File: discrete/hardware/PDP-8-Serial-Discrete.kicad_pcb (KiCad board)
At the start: 2 copper layers, 125.2 x 61.9 mm, 103 parts, among them J1 Screw_Terminal_01x06, J2 DE9_Socket_MountingHoles, J3 FlipChip_01x18, Q1 2N5551, Q10 2N5401, Q11 2N5401, Q12 2N5551, Q13 2N5401, Q14 2N5551, Q15 2N5401, Q16 2N5551, Q17 2N5401, Q2 2N5401, Q3 2N5401, Q4 2N5401, Q5 2N5551, Q6 2N5401, Q7 2N5551, Q8 2N5401, Q9 2N5551

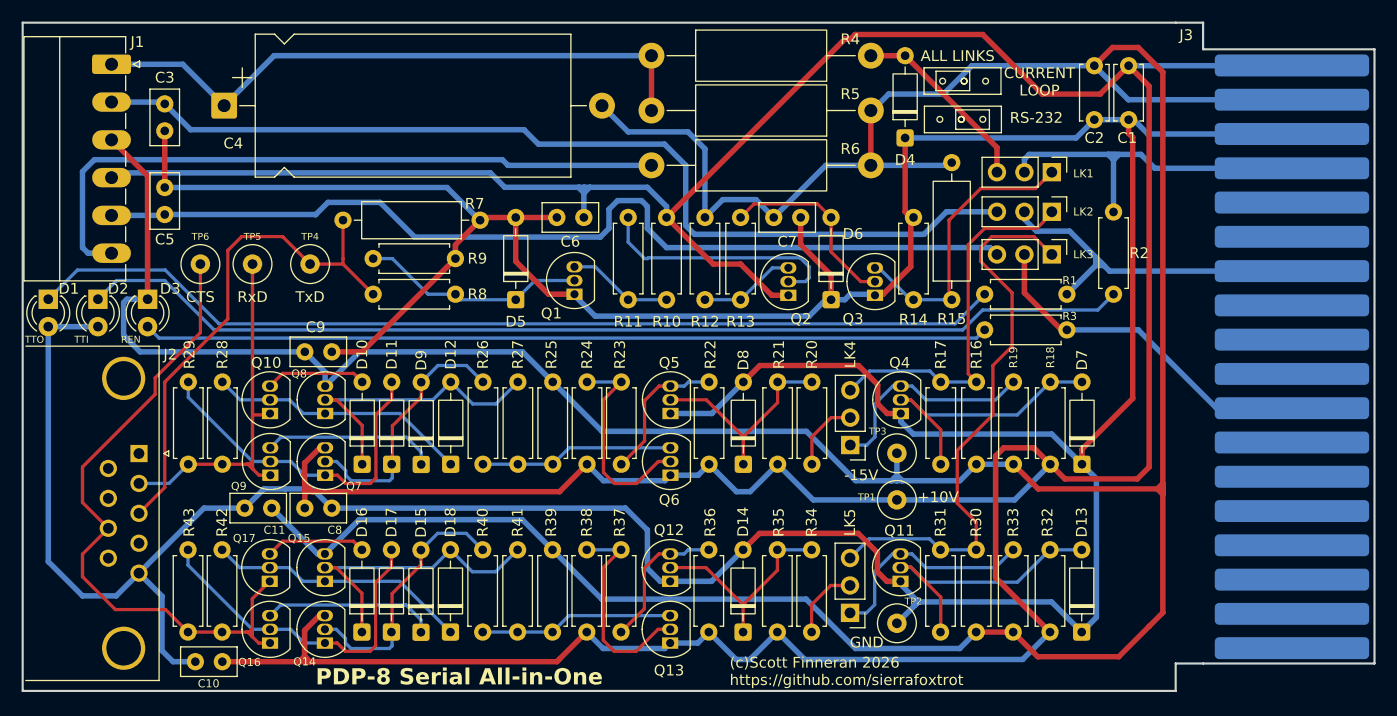
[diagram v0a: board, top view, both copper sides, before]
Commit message: PCB cleanup
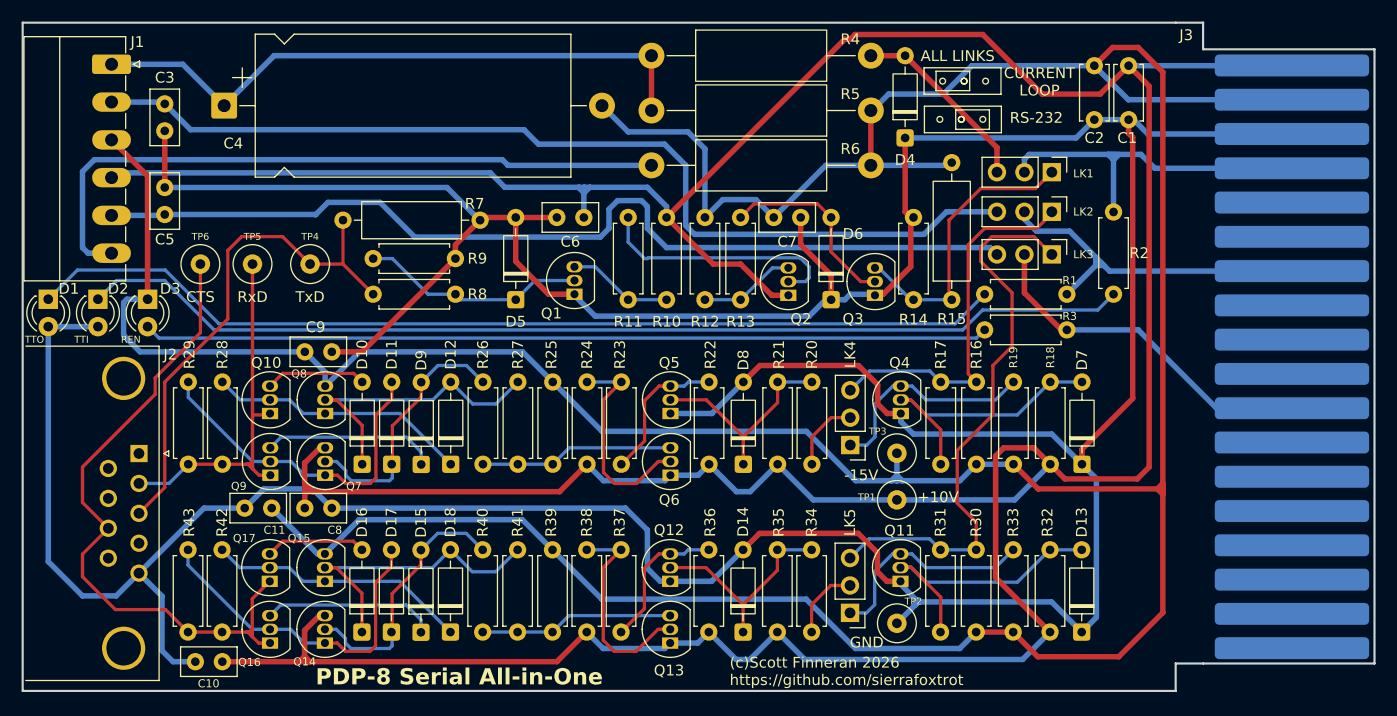
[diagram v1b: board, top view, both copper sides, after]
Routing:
- net +10V: track 388.0 -> 387.4 mm
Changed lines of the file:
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@@
 	)
 	(segment
-		(start 108.966 130.302)
-		(end 106.974 130.302)
+		(start 106.974 130.302)
+		(end 111.486 130.302)
 		(width 0.508)
 		(layer "B.Cu")
@@
 	)
 	(segment
-		(start 181.292501 126.555499)
-		(end 182.753 128.015999)
-		(width 0.508)
-		(layer "B.Cu")
-		(net 1)
-	)
-	(segment
 		(start 159.004 112.776)
 		(end 157.48 114.3)
@@
 	)
 	(segment
-		(start 181.267704 142.101005)
+		(start 179.934205 140.767506)
 		(end 182.728203 143.561505)
 		(width 0.508)
@@
 	)
 	(segment
-		(start 179.934205 140.767506)
-		(end 181.267704 142.101005)
-		(width 0.508)
-		(layer "B.Cu")
-		(net 1)
-	)
-	(segment
 		(start 140.462 132.08)
 		(end 113.264 132.08)
@@
 	)
 	(segment
-		(start 111.486 130.302)
-		(end 108.966 130.302)
-		(width 0.508)
-		(layer "B.Cu")
-		(net 1)
-	)
-	(segment
 		(start 163.322 112.268)
 		(end 161.29 112.268)
@@
 	(segment
 		(start 179.959002 125.222)
-		(end 181.292501 126.555499)
+		(end 182.753 128.015999)
 		(width 0.508)
 		(layer "B.Cu")
@@
 	)
 	(segment
-		(start 110.744 145.288)
+		(start 110.744 145.796)
 		(end 110.744 143.403274)
 		(width 0.508)
@@
 	(segment
 		(start 134.111999 146.304)
-		(end 134.365999 146.05)
+		(end 136.906 143.509999)
 		(width 0.508)
 		(layer "F.Cu")
@@
 	)
 	(segment
-		(start 110.744 145.796)
-		(end 110.744 145.288)
-		(width 0.508)
-		(layer "F.Cu")
-		(net 2)
-	)
-	(segment
 		(start 134.365999 130.556)
 		(end 111.506 130.556)
@@
 	)
 	(segment
-		(start 136.906 143.509999)
-		(end 134.365999 146.05)
-		(width 0.508)
-		(layer "F.Cu")
-		(net 2)
-	)
-	(segment
 		(start 110.744 127.909274)
 		(end 112.161275 126.491999)
@@
 	)
 	(segment
-		(start 154.559 128.015999)
-		(end 154.559 128.143)
-		(width 0.508)
-		(layer "B.Cu")
-		(net 2)
-	)
-	(segment
 		(start 142.494 102.362)
 		(end 144.272 104.14)
@@
 	)
 	(segment
-		(start 201.922 91.353)
-		(end 202.2 91.075)
-		(width 0.508)
-		(layer "B.Cu")
-		(net 2)
-	)
-	(segment
-		(start 154.534203 143.561505)
-		(end 154.534203 143.688506)
-		(width 0.508)
-		(layer "B.Cu")
-		(net 2)
-	)
-	(segment
 		(start 144.123999 129.54)
 		(end 138.430001 129.54)
@@
 	)
 	(segment
-		(start 188.976 143.028709)
-		(end 186.157203 145.847506)
-		(width 0.508)
-		(layer "F.Cu")
-		(net 3)
-	)
-	(segment
-		(start 190.246 141.758709)
-		(end 188.976 143.028709)
+		(start 186.157203 145.847506)
+		(end 190.246 141.758709)
 		(width 0.508)
 		(layer "F.Cu")
@@
 	)
 	(segment
-		(start 170.18 100.33)
-		(end 170.434 100.076)
-		(width 0.508)
-		(layer "B.Cu")
-		(net 3)
-	)
-	(segment
 		(start 187.047 94.25)
 		(end 202.2 94.25)
@@
 	)
 	(segment
-		(start 124.46 120.395999)
-		(end 124.46 120.65)
-		(width 0.3048)
-		(layer "F.Cu")
-		(net 12)
-	)
-	(segment
 		(start 116.078 124.421199)
 		(end 113.7038 122.046999)
@@
 	)
 	(segment
-		(start 124.435203 135.941505)
-		(end 124.435203 136.195506)
-		(width 0.3048)
-		(layer "F.Cu")
-		(net 18)
-	)
-	(segment
 		(start 113.679003 137.592505)
 		(end 112.624203 137.592505)
@@
 	(segment
 		(start 105.893203 143.307506)
-		(end 105.893204 143.307505)
+		(end 107.544203 143.307505)
 		(width 0.3048)
 		(layer "B.Cu")
@@
 	)
 	(segment
-		(start 105.893204 143.307505)
-		(end 107.544203 143.307505)
-		(width 0.3048)
-		(layer "B.Cu")
-		(net 20)
-	)
-	(segment
 		(start 110.719202 144.577505)
 		(end 109.449203 143.307506)
@@
 	)
 	(segment
-		(start 114.3 108.966)
+		(start 114.3 109.474)
 		(end 114.3 105.41)
 		(width 0.3048)
@@
 		(width 0.3048)
 		(layer "F.Cu")
-		(net 23)
-	)
-	(segment
-		(start 114.3 109.474)
-		(end 114.3 108.966)
-		(width 0.3048)
-		(layer "F.Cu")
